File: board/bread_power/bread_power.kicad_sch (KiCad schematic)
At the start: 23 parts, among them J1 USB_C_Receptacle_PowerOnly_6P, U1 TPS61022, U2 BQ24073RGT

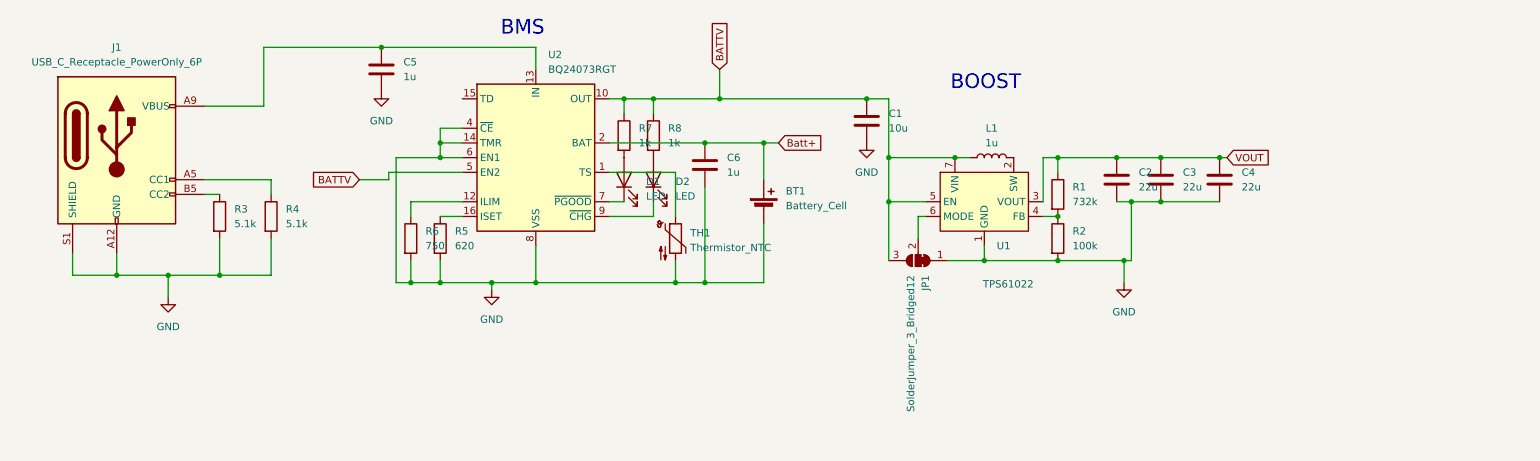
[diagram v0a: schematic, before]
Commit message: Updates for part annotations.
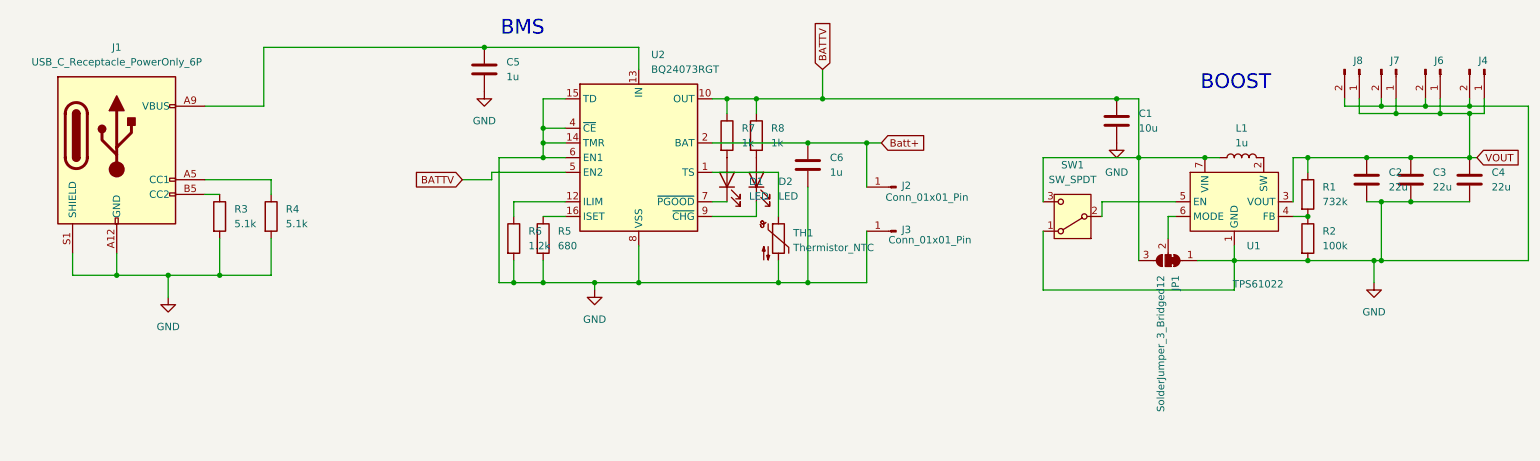
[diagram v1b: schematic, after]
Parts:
- removed BT1: Battery_Cell, Battery:BatteryClip_Keystone_54_D16-19mm, symbol Device:Battery_Cell
- added J2, J3: Conn_01x01_Pin, Battery:BatteryClip_Keystone_54_D16-19mm, symbol Connector:Conn_01x01_Pin
- added J4, J6, J7, J8: Conn_01x02_Pin, symbol Connector:Conn_01x02_Pin
- added SW1: SW_SPDT, Button_Switch_SMD:SW_SPDT_PCM12, symbol Switch:SW_SPDT
- C1, C5, C6: footprint (none) -> Capacitor_SMD:C_0805_2012Metric
- C2, C3, C4: footprint (none) -> Capacitor_SMD:C_1206_3216Metric
- D1, D2: footprint (none) -> LED_SMD:LED_0805_2012Metric
- JP1: footprint (none) -> Jumper:SolderJumper-3_P1.3mm_Bridged12_RoundedPad1.0x1.5mm
- R1, R2, R3, R4, R7, R8: footprint (none) -> Resistor_SMD:R_0402_1005Metric
- R5: value 620 -> 680; footprint (none) -> Resistor_SMD:R_0603_1608Metric
- R6: value 750 -> 1.2k; footprint (none) -> Resistor_SMD:R_0603_1608Metric
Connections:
- net BATTV: now also SW1.3 (C); no longer U1.5 (EN)
- net Batt+: now also J2.1 (Pin_1)
- net GND: now also U2.15 (TD), J3.1 (Pin_1), J4.2 (Pin_2), J6.2 (Pin_2), J7.2 (Pin_2), J8.2 (Pin_2), SW1.1 (A)
- net VOUT: now also J4.1 (Pin_1), J6.1 (Pin_1), J7.1 (Pin_1), J8.1 (Pin_1)
- new net: SW1.2 (B), U1.5 (EN)
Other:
- moved on the sheet: C1, C2, C3, C4, C5, C6, D1, D2, JP1, L1, R1, R2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
